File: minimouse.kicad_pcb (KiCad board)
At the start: 2 copper layers, 90 x 85 mm, 22 parts, among them J1 Conn_ARM_JTAG_SWD_10, J5 Conn_01x02, M1 N20_encoder, M2 N20_encoder, U1 STM32F030C8Tx, U4 HC-SR04

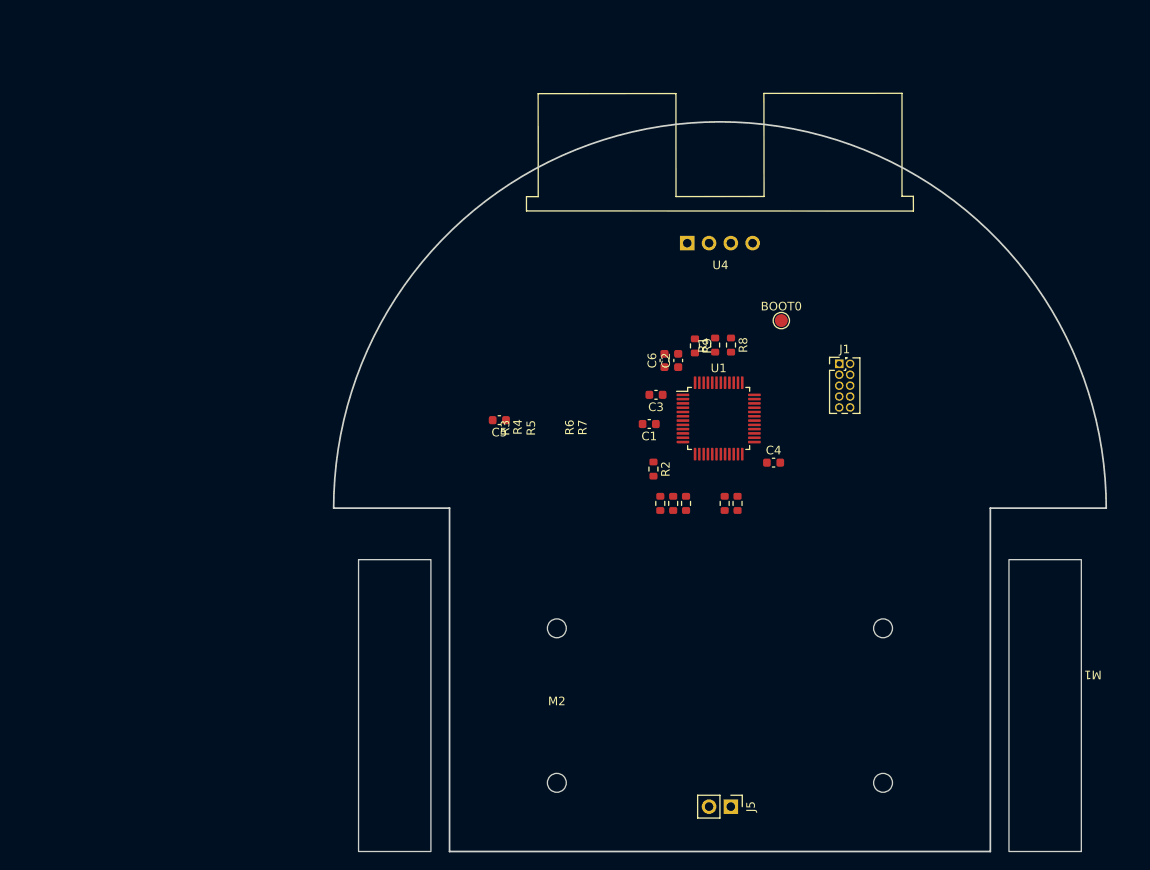
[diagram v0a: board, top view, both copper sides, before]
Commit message: TP3
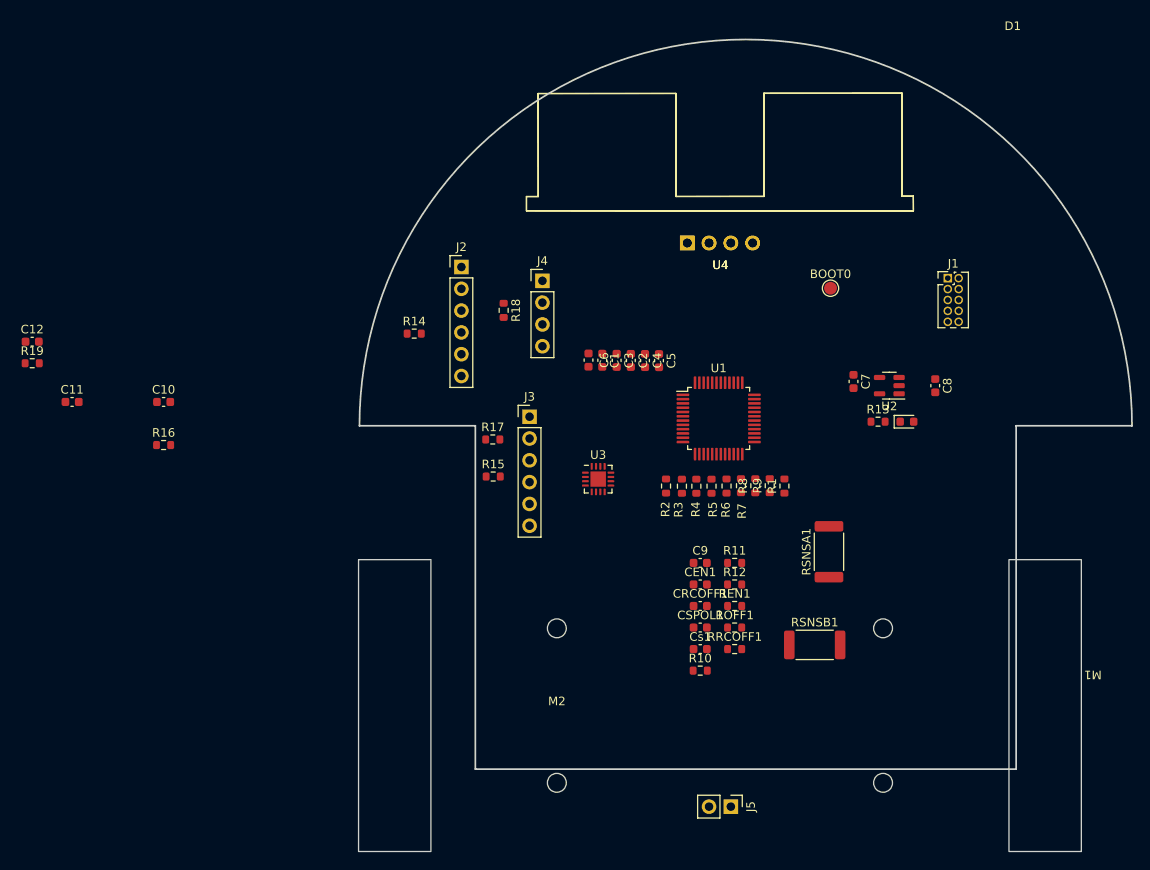
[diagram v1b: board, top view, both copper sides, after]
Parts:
- added C10: 2.2 uF, Capacitor_SMD:C_0603_1608Metric, F.Cu at (85.2, 87.6)
- added C11: 2.2 uF, Capacitor_SMD:C_0603_1608Metric, F.Cu at (74.5, 87.6)
- added C12: 2.2uF, Capacitor_SMD:C_0603_1608Metric, F.Cu at (69.9, 80.6)
- added C7: 1uF, Capacitor_SMD:C_0603_1608Metric, F.Cu at (165.6, 85.2)
- added C8: 1uF, Capacitor_SMD:C_0603_1608Metric, F.Cu at (175.1, 85.7)
- added C9: C, Capacitor_SMD:C_0603_1608Metric, F.Cu at (147.7, 106.4)
- added CEN1: 10nF, Capacitor_SMD:C_0603_1608Metric, F.Cu at (147.7, 108.9)
- added CRCOFF1: 22nF, Capacitor_SMD:C_0603_1608Metric, F.Cu at (147.7, 111.4)
- added CSPOL1: 22uF, Capacitor_SMD:C_0603_1608Metric, F.Cu at (147.7, 113.9)
- added Cs1: 2.2uF, Capacitor_SMD:C_0603_1608Metric, F.Cu at (147.7, 116.4)
- added D1: LED, LED_SMD:LED_0603_1608Metric, F.Cu at (171.8, 89.9)
- added J2: Conn_01x06, Connector_PinHeader_2.54mm:PinHeader_1x06_P2.54mm_Vertical, F.Cu at (119.9, 71.9)
- added J3: Conn_01x06, Connector_PinHeader_2.54mm:PinHeader_1x06_P2.54mm_Vertical, F.Cu at (127.8, 89.3)
- added J4: Conn_01x04, Connector_PinHeader_2.54mm:PinHeader_1x04_P2.54mm_Vertical, F.Cu at (129.3, 73.5)
- added R10: 10k, Resistor_SMD:R_0603_1608Metric, F.Cu at (147.7, 118.9)
- added R11: 10k, Resistor_SMD:R_0603_1608Metric, F.Cu at (151.7, 106.4)
- added R12: R, Resistor_SMD:R_0603_1608Metric, F.Cu at (151.7, 108.9)
- added R13: R, Resistor_SMD:R_0603_1608Metric, F.Cu at (168.4, 89.9)
- added R14: 100, Resistor_SMD:R_0603_1608Metric, F.Cu at (114.4, 79.7)
- added R15: 100, Resistor_SMD:R_0603_1608Metric, F.Cu at (123.6, 96.3)
- added R16: 10, Resistor_SMD:R_0603_1608Metric, F.Cu at (85.2, 92.7)
- added R17: 10, Resistor_SMD:R_0603_1608Metric, F.Cu at (123.5, 92.0)
- added R18: 100, Resistor_SMD:R_0603_1608Metric, F.Cu at (124.8, 77.0)
- added R19: 100, Resistor_SMD:R_0603_1608Metric, F.Cu at (69.9, 83.1)
- added REN1: 18k, Resistor_SMD:R_0603_1608Metric, F.Cu at (151.7, 111.4)
- added ROFF1: 47k, Resistor_SMD:R_0603_1608Metric, F.Cu at (151.7, 113.9)
- added RRCOFF1: 1k, Resistor_SMD:R_0603_1608Metric, F.Cu at (151.7, 116.4)
- added RSNSA1: 330m, Resistor_SMD:R_2512_6332Metric, F.Cu at (162.7, 105.1)
- added RSNSB1: 330m, Resistor_SMD:R_2512_6332Metric, F.Cu at (161.0, 115.9)
- added U2: LP5907MFX-1.2, Package_TO_SOT_SMD:SOT-23-5, F.Cu at (169.7, 85.7)
- added U3: STSPIN240, Package_DFN_QFN:VQFN-16-1EP_3x3mm_P0.5mm_EP1.8x1.8mm, F.Cu at (135.8, 96.6)
- added U4: HC-SR04, minimouse:HC-SR04, F.Cu at (150.0, 69.1)
- moved C5 19.9 mm to (142.9, 82.8), turned to -90 degrees
- moved C4 19.1 mm to (141.3, 82.8), turned to -90 degrees
- moved R9 18.5 mm to (155.8, 97.4), turned to 90 degrees
- moved R1 18.3 mm to (157.5, 97.4)
- moved R8 16.6 mm to (154.1, 97.4), turned to 90 degrees
- moved J1 16.1 mm to (176.5, 73.2)
- moved C1 9.22 mm to (136.3, 82.8), turned to -90 degrees
- moved C6 8.85 mm to (134.7, 82.8), turned to -90 degrees
- moved BOOT0 6.86 mm to (162.9, 74.4)
- moved C3 6.09 mm to (138.0, 82.8), turned to -90 degrees
- moved C2 5.52 mm to (139.6, 82.8), turned to -90 degrees
- moved R5 3.58 mm to (149.0, 97.4)
- moved R4 3.36 mm to (147.2, 97.4)
- moved R3 3.22 mm to (145.6, 97.4)
- moved R2 2.46 mm to (143.7, 97.4)
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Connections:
- R6 pad 1: /mcu/OUT_B0 -> /motor_control/STBY/RESET
- R8 pad 1: /mcu/UART1_TX -> /external_uart/EXT_UART_RX
- U1 pad 43: /mcu/UART1_RX -> /external_uart/EXT_UART_TX
